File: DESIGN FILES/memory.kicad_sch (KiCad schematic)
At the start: 29 parts, among them J1 TF-15x15, Q1 IRLML6401, U2 IS42S16160J-6BLI, U3 IS25WP064A-JBLE

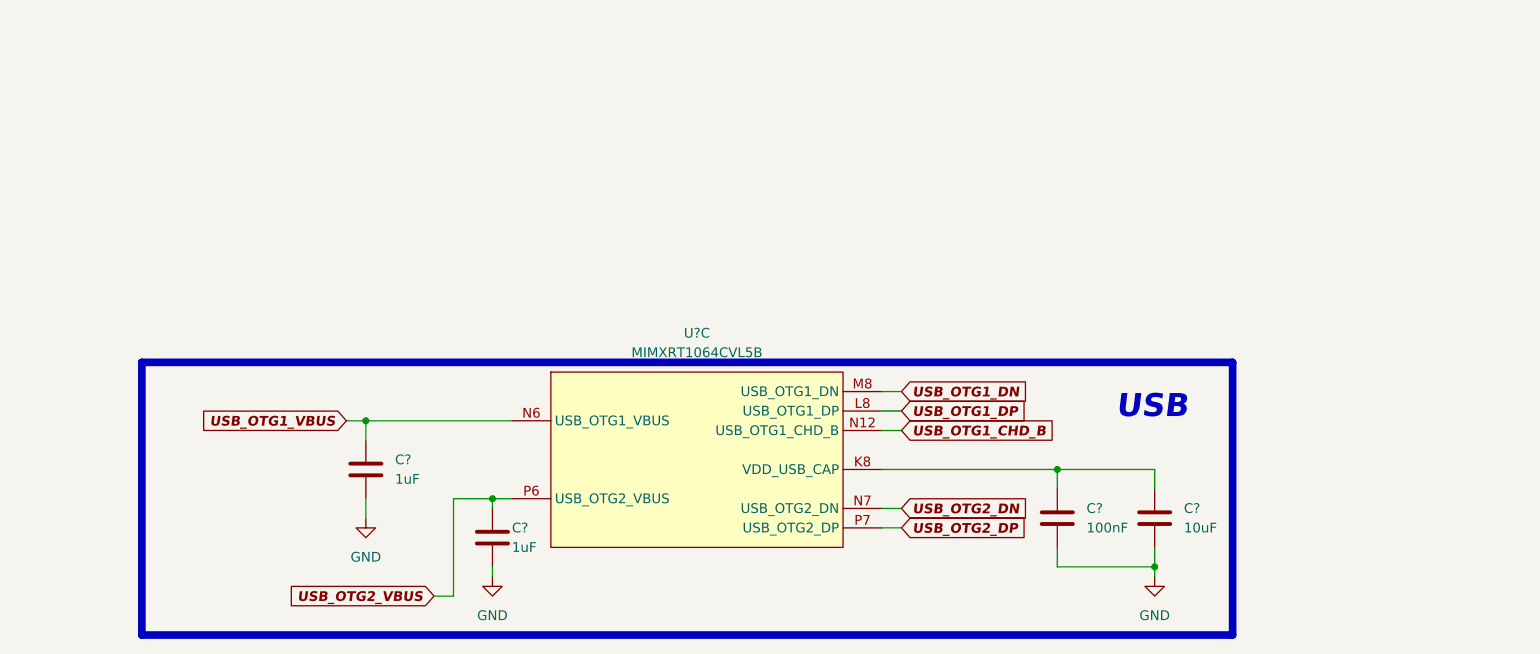
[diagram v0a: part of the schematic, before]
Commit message: schematic edit
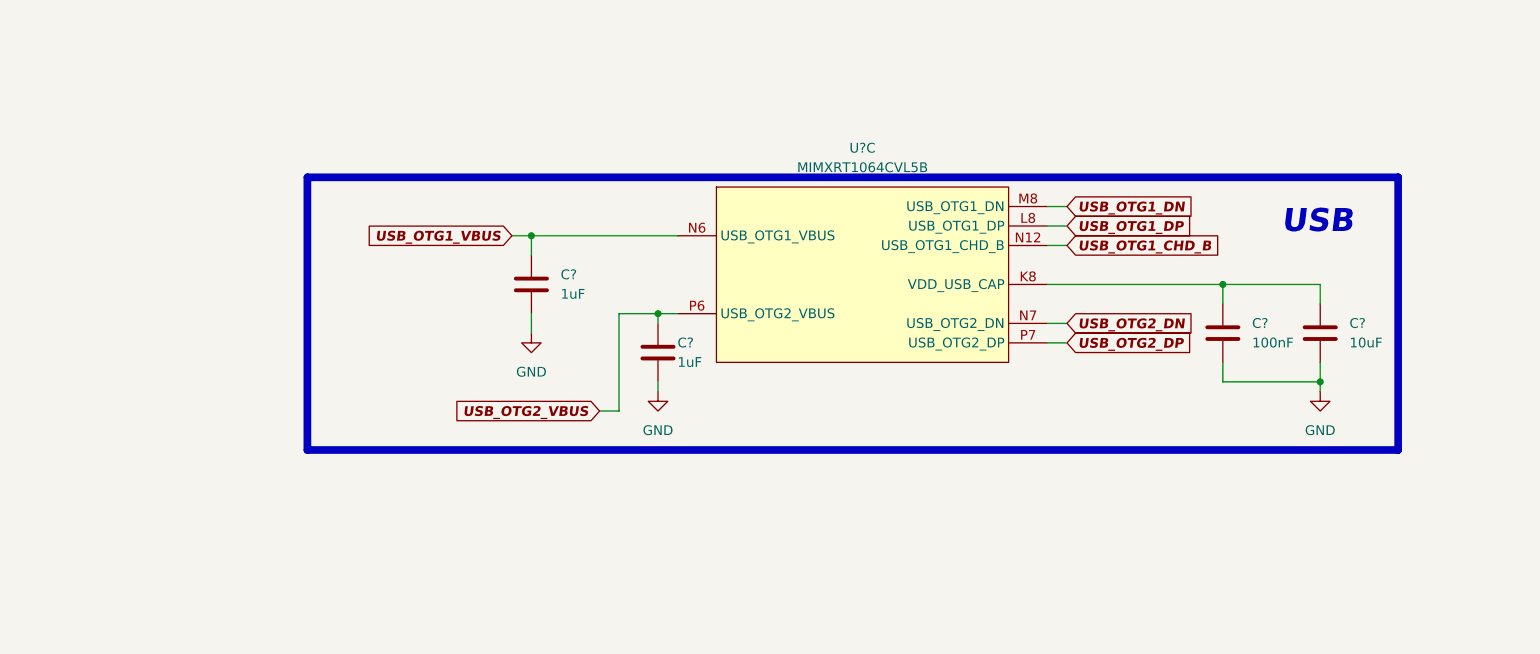
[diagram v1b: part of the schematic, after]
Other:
- moved on the sheet: C?, U?C

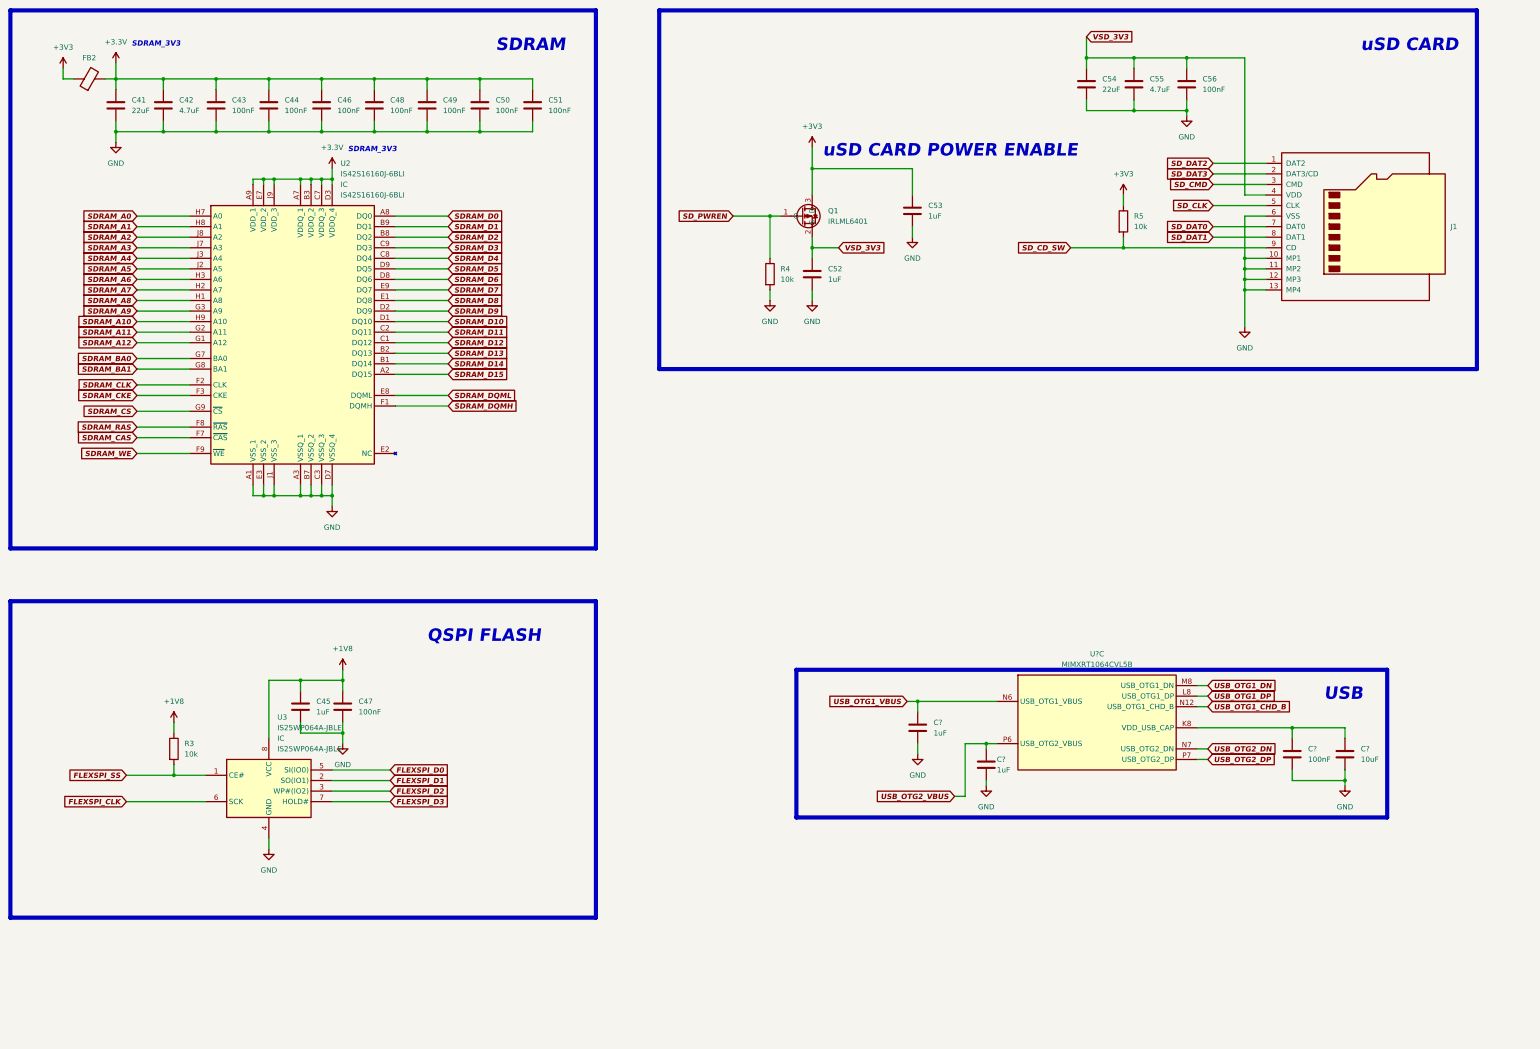
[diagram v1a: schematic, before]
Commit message: schematic changes
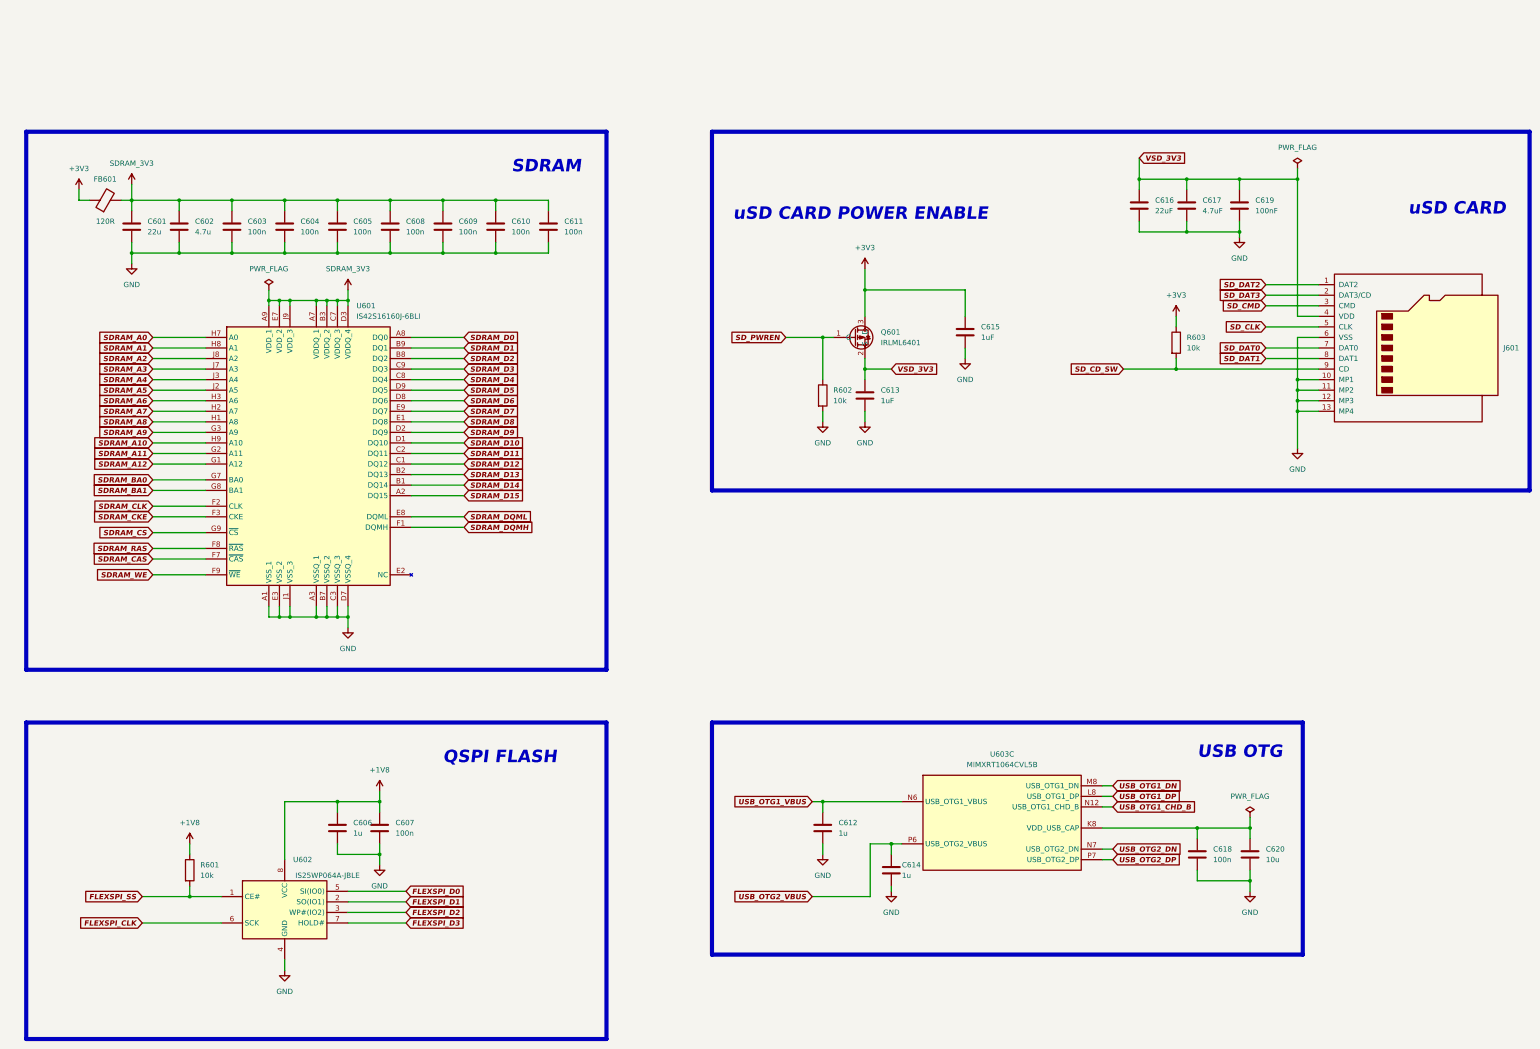
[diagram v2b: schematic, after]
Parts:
- C601: renamed from C41; value 22uF -> 22u
- C602: renamed from C42; value 4.7uF -> 4.7u
- C603: renamed from C43; value 100nF -> 100n
- C604: renamed from C44; value 100nF -> 100n
- C605: renamed from C46; value 100nF -> 100n
- C606: renamed from C45; value 1uF -> 1u
- C607: renamed from C47; value 100nF -> 100n
- C608: renamed from C48; value 100nF -> 100n
- C609: renamed from C49; value 100nF -> 100n
- C610: renamed from C50; value 100nF -> 100n
- C611: renamed from C51; value 100nF -> 100n
- C612, C614: renamed from C?; value 1uF -> 1u
- C618: renamed from C?; value 100nF -> 100n
- C620: renamed from C?; value 10uF -> 10u
- FB601: renamed from FB2; value BLM18AG121SN1D -> 120R
- gave numbers to parts that had none: 1
- renumbered C52 to C613, C53 to C615, C54 to C616, C55 to C617, C56 to C619, J1 to J601, Q1 to Q601, R3 to R601, R4 to R602, R5 to R603, U2 to U601, U3 to U602
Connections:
- net +3.3V renamed SDRAM_3V3
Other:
- note added: "USB OTG"
- note removed: "SDRAM_3V3"
- note removed: "USB"
- moved on the sheet: C601, C602, C603, C604, C605, C606, C607, C608, C609, C610, C611, C612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
